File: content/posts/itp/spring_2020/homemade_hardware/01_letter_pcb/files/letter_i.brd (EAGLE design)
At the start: 43.7 x 70 mm, 61 parts

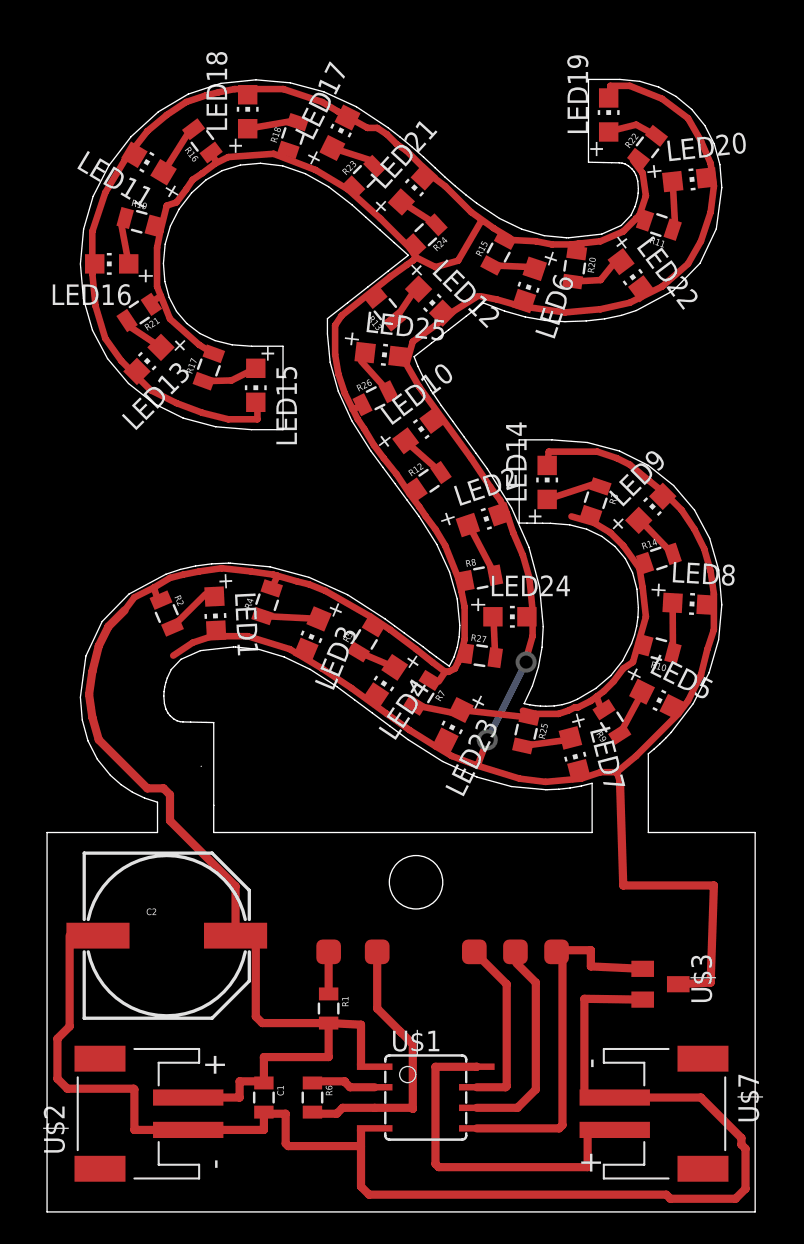
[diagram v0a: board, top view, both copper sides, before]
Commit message: hmhw 01 - new files
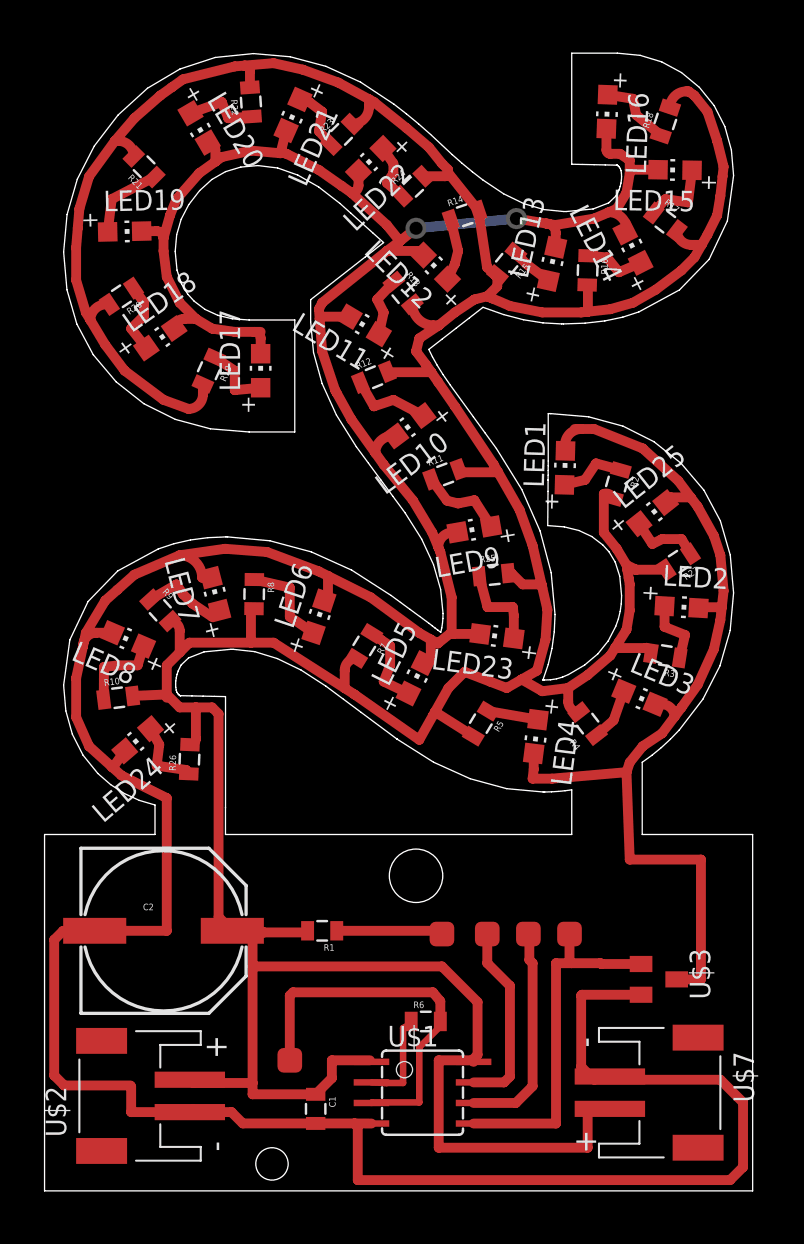
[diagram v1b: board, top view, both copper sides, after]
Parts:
- moved LED8 34.8 mm to (10.6, 40.8), turned to 66.8 degrees
- moved R10 33.5 mm to (10.0, 37.2), turned to 7.1 degrees
- moved LED16 32.0 mm to (40.2, 73.4), turned to 177.9 degrees
- moved LED19 30.8 mm to (10.4, 66.0), turned to 271.3 degrees
- moved LED20 30.5 mm to (15.0, 72.4), turned to 210.4 degrees
- moved R17 29.6 mm to (43.8, 66.6), turned to 322.6 degrees
- moved LED15 29.1 mm to (44.4, 69.8), turned to 89.1 degrees
- moved R2 28.9 mm to (40.8, 50.4), turned to 254.1 degrees
- moved R9 28.7 mm to (12.6, 42.6), turned to 312.1 degrees
- moved R20 28.1 mm to (10.2, 62.0), turned to 213.7 degrees
- moved LED13 25.6 mm to (36.8, 64.0), turned to 347.4 degrees
- moved R16 25.1 mm to (39.0, 63.6), turned to 268.3 degrees
- moved R26 25.1 mm to (14.4, 33.4), turned to 87.6 degrees
- moved R22 24.7 mm to (18.2, 74.0), turned to 93.9 degrees
- moved R14 24.4 mm to (31.4, 67.0)
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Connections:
- net N$3 renamed GND
- net N$4 renamed PWR
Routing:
- net GND: track 191.8 -> 308.4 mm, vias 0 -> 2
- net PWR: track 205.5 -> 285.1 mm
- net N$23: track 55.4 -> 4.53 mm
- net N$20: track 29.1 -> 3.84 mm
- net N$22: track 23.7 -> 3.81 mm
- net N$10: track 16.5 -> 23.4 mm
- net N$9: track 0.00 -> 5.82 mm
- net N$1: track 5.37 -> 0.00 mm, vias 1 -> 0
- net N$8: track 0.00 -> 5.34 mm
- net N$17: track 0.00 -> 5.28 mm
- net N$18: track 0.00 -> 5.03 mm
- net N$27: track 0.00 -> 5.01 mm
- net N$32: track 0.00 -> 4.56 mm
- net N$11: track 2.10 -> 6.58 mm
- net N$33: track 0.00 -> 4.43 mm
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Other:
- board size 43.7 x 70 mm -> 43.7 x 70.3 mm
